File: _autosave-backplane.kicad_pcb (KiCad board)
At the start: 4 copper layers, 110 x 90 mm, 57 parts, among them IC1 SiC437AED-T1-GE3, J1 46010-0622, J2 46010-0622, J4 212520-1006, J5 XT60PW-F

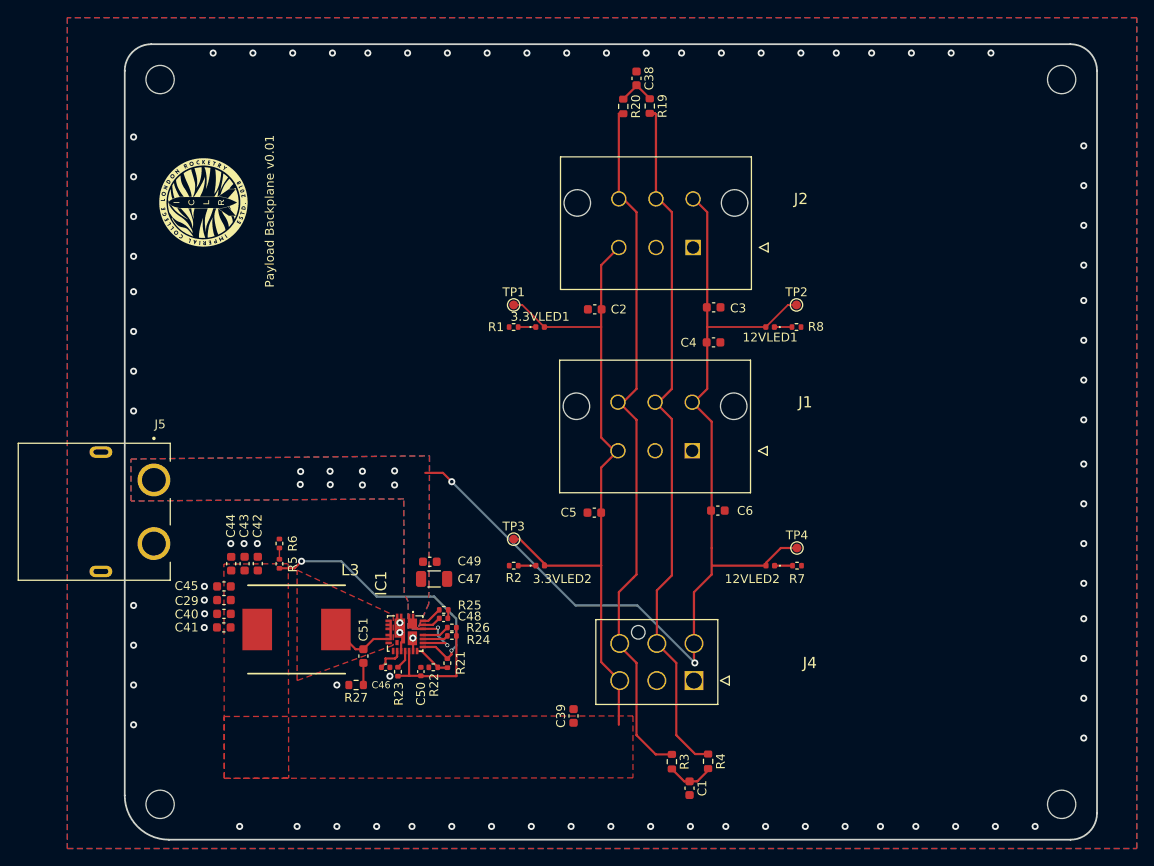
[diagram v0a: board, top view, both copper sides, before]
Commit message: filleted
to add switches then next review
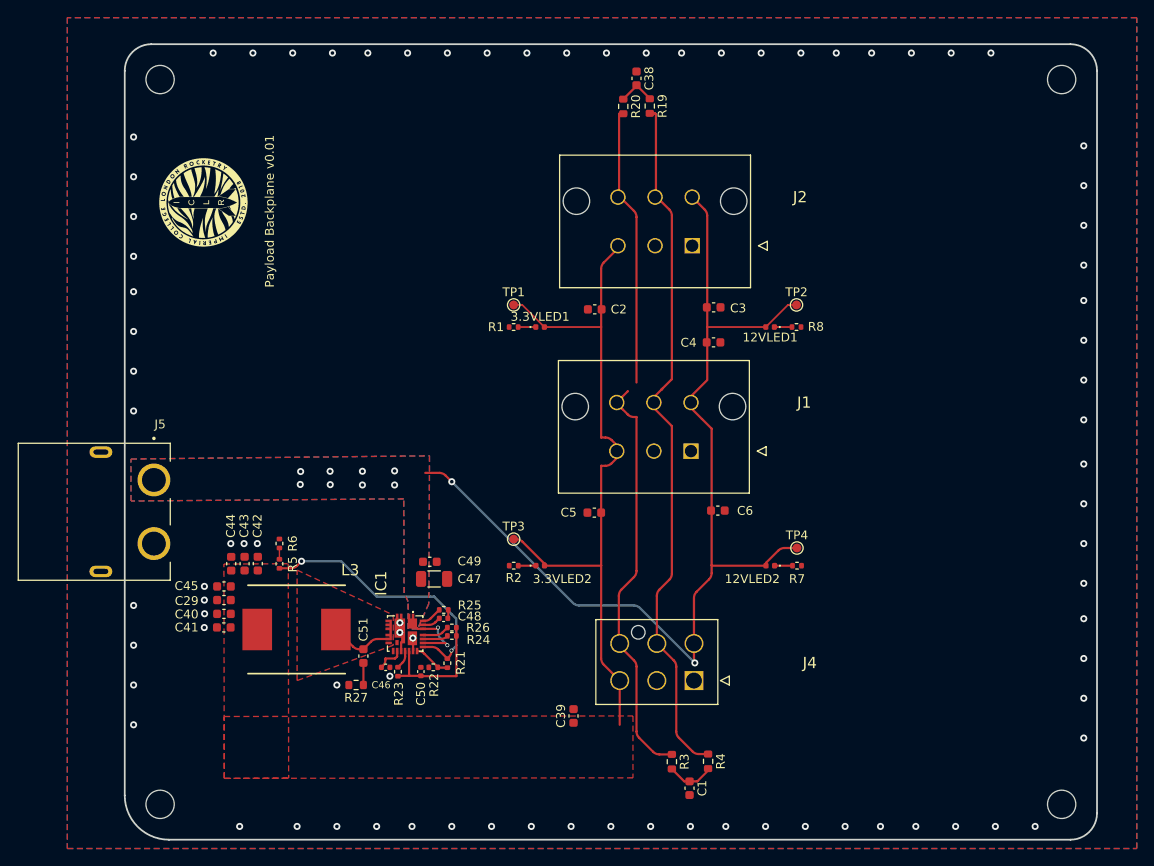
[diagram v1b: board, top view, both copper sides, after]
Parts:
- moved J2 0.22 mm to (151.2, 80.8)
- moved J1 0.14 mm to (151.1, 104.0)
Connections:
- C47 pad 1: Net-(IC1-EN) -> +12V
- C49 pad 1: Net-(IC1-EN) -> +12V
- IC1 pad 1: Net-(IC1-EN) -> +12V
- IC1 pad 19: Net-(IC1-EN) -> +12V
- IC1 pad 2: Net-(IC1-EN) -> +12V
- IC1 pad 22: Net-(IC1-EN) -> +12V
- IC1 pad 26: Net-(IC1-EN) -> +12V
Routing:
- net Net-(IC1-EN): track 9.01 -> 0.00 mm, vias 2 -> 0
- net +12V: track 117.3 -> 125.6 mm, vias 10 -> 12
- net CAN_H: track 80.6 -> 78.2 mm
- net +3.3V: track 79.6 -> 80.3 mm
- net GND: track 3.26 -> 2.76 mm
